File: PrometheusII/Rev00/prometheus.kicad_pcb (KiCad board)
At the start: 4 copper layers, 223.5 x 222.3 mm, 194 parts, among them J1 0878311420, J10 Conn_02x02_Odd_Even, J11 Conn_02x02_Odd_Even, J16 Conn_02x07_Odd_Even, J17 Conn_02x07_Odd_Even, J18 Conn_02x07_Odd_Even, J19 Conn_02x07_Odd_Even, J2 Conn_02x08_Odd_Even, J3 Conn_02x02_Odd_Even, J4 Conn_02x02_Odd_Even, J5 Conn_02x05_Odd_Even, J6 Conn_02x05_Odd_Even, Q1 MMBF4391, Q2 MMBF4391, Q3 BSS138, Q4 BSS84, Q6 BSS84, U1 Teensy4.0_NoSD, U10 74LVC2G157, U2 XC2C32A_LFSR, U3 XC2C32A_LFSR, U4 TL072CDR, U5 TL072CDR, U6 MIC5504-1.8YM5, U7 MCP6002-xMS, U8 TL072CDR, U9 MCP6002-xMS

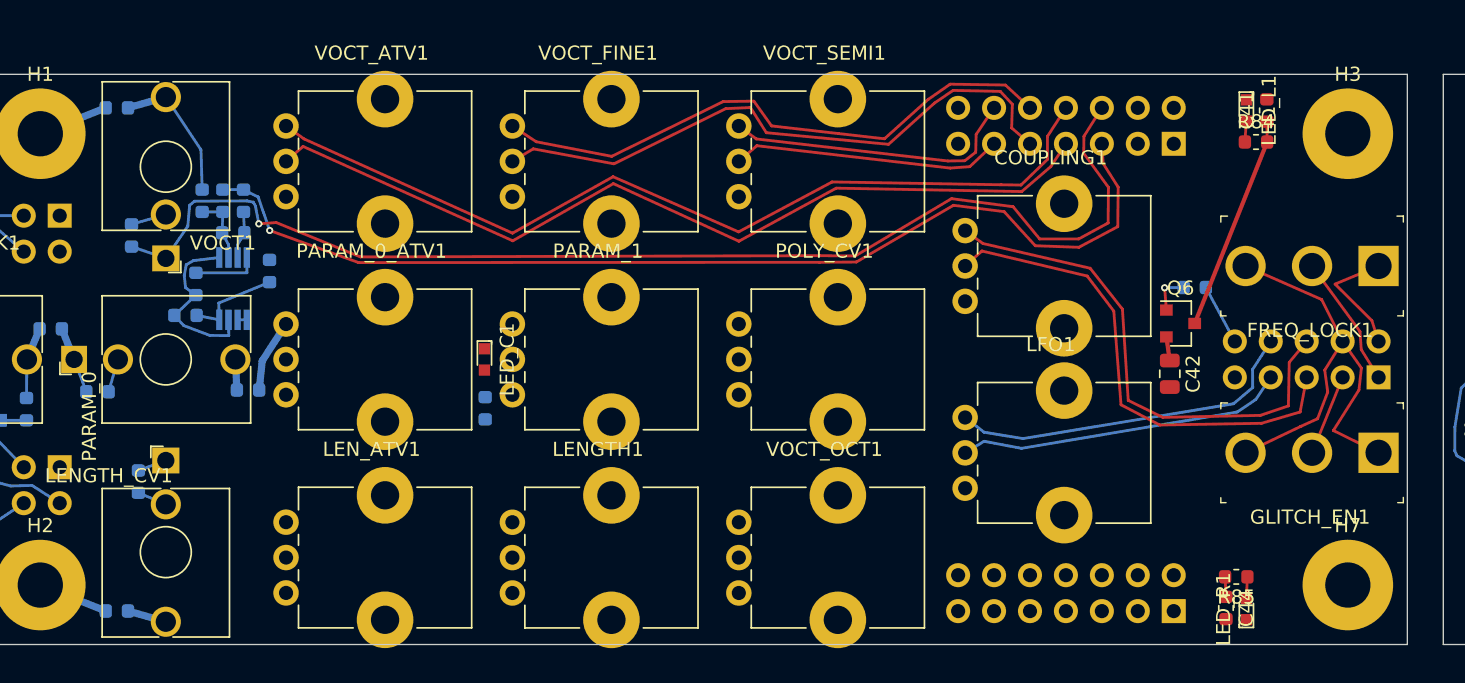
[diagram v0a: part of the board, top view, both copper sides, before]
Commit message: checkpoint
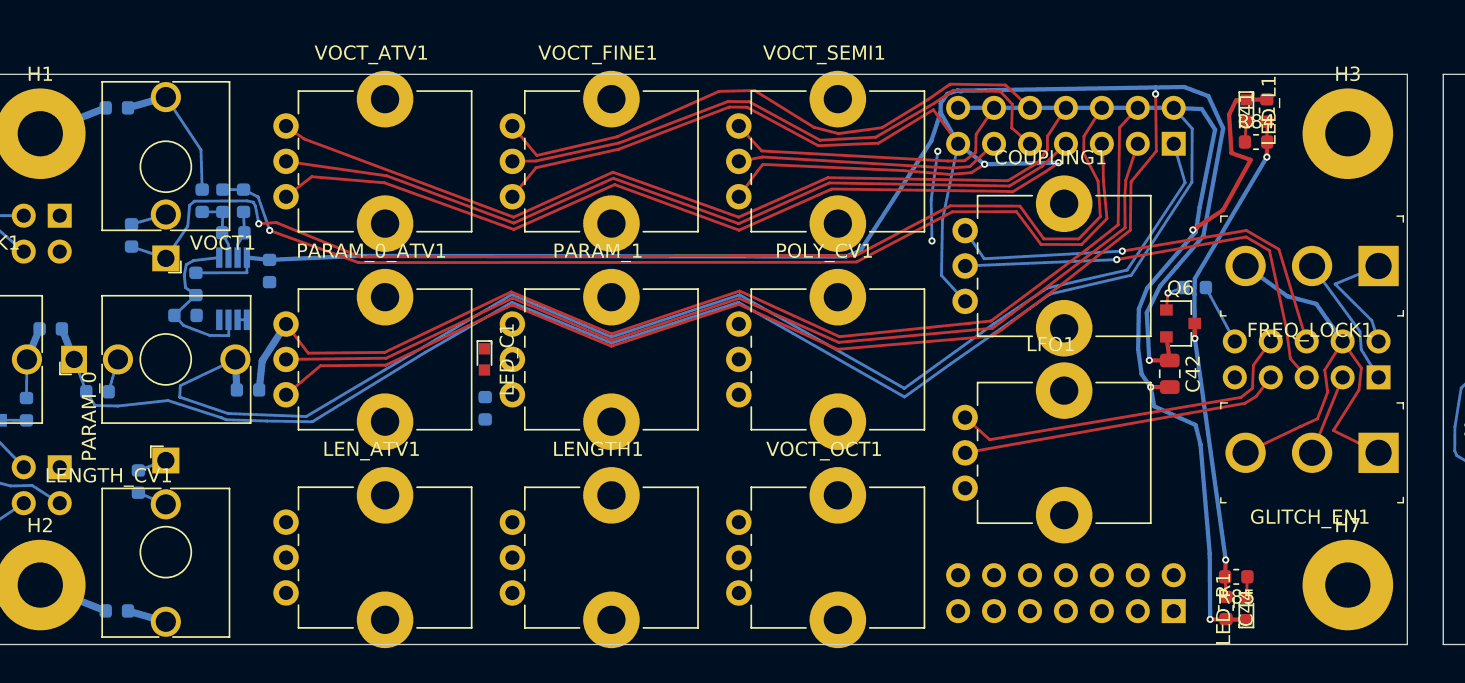
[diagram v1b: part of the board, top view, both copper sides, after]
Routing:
- net +3V3: track 299.2 -> 607.3 mm, vias 6 -> 10
- net GND: track 693.9 -> 929.8 mm, vias 92 -> 98
- net /PARAM_0_CV_P: track 2.16 -> 92.3 mm
- net /PARAM_0_P: track 0.00 -> 70.5 mm
- net Net-(C41-Pad1): track 16.7 -> 36.2 mm, vias 0 -> 3
- net /CV_FILT_P: track 34.6 -> 31.5 mm, vias 0 -> 1
- net /VOCT_ATV_P: track 61.4 -> 58.7 mm
- net /VOCT_FINE_P: track 42.8 -> 41.4 mm
- net /VOCT_CV_P: track 74.2 -> 72.8 mm
- net Net-(Q6-Pad1): track 2.92 -> 2.38 mm
